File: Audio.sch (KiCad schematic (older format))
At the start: 53 parts, among them J5 PJ-3270, J6 PJ-3270, J7 PJ-3270, U6 SSM2603, Y1 12.288Mhz

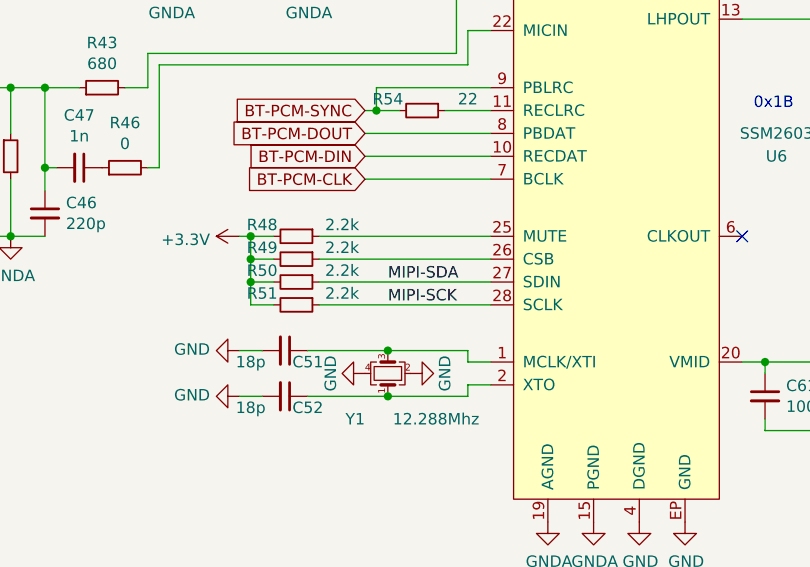
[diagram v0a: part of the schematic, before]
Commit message: update
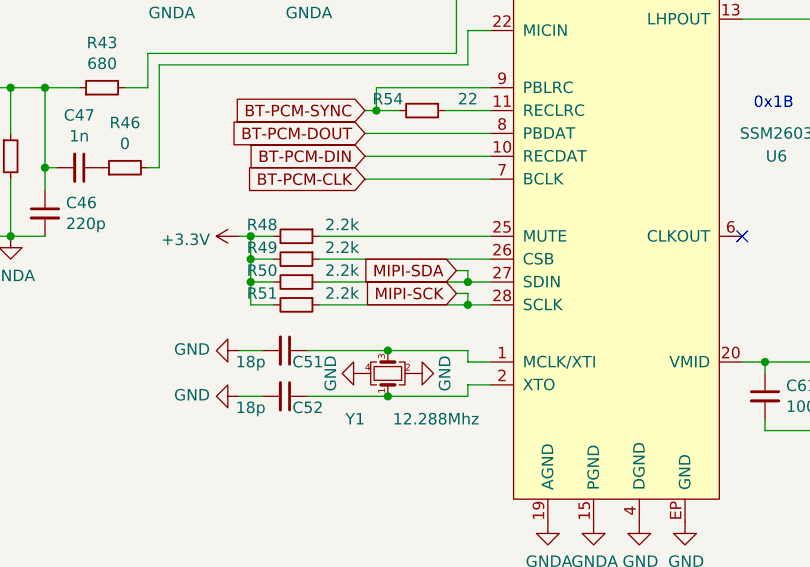
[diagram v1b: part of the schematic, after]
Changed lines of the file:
@@
 Connection ~ 4150 4750
 Wire Wire Line
-	4450 4750 5200 4750
-Wire Wire Line
-	5200 4850 4450 4850
-Text Label 4750 4850 0    50   ~ 0
-MIPI-SCK
-Text Label 4750 4750 0    50   ~ 0
-MIPI-SDA
+	4450 4750 5100 4750
+Wire Wire Line
+	5200 4850 5100 4850
 $Comp
 L Device:R_Small R?
@@
 	1    0    0    -1
 $EndComp
+Text GLabel 5050 4700 0    50   Input ~ 0
+MIPI-SDA
+Text GLabel 5050 4800 0    50   Input ~ 0
+MIPI-SCK
+Wire Wire Line
+	5050 4800 5100 4800
+Wire Wire Line
+	5100 4800 5100 4850
+Connection ~ 5100 4850
+Wire Wire Line
+	5100 4850 4450 4850
+Wire Wire Line
+	5050 4700 5100 4700
+Wire Wire Line
+	5100 4700 5100 4750
+Connection ~ 5100 4750
+Wire Wire Line
+	5100 4750 5200 4750
 $EndSCHEMATC
